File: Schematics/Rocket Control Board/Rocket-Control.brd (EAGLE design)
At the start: 100 x 80 mm, 37 parts

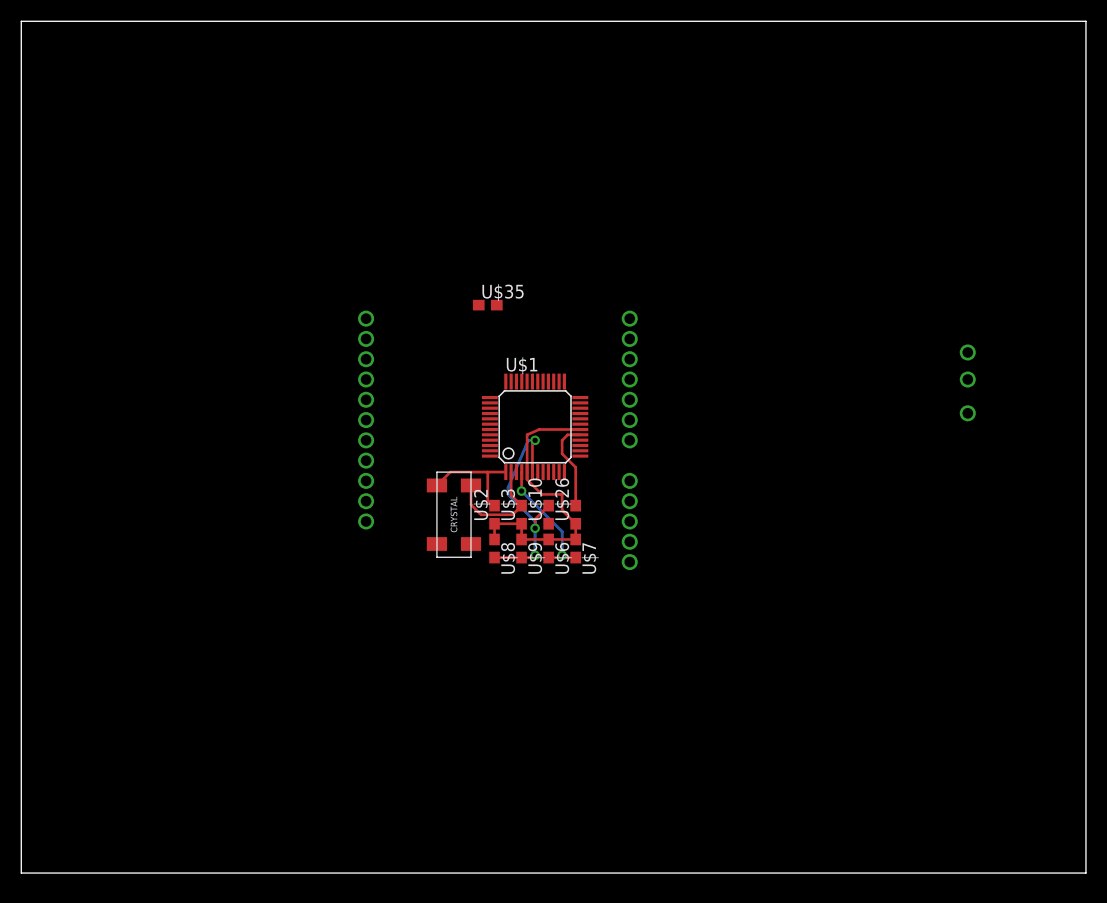
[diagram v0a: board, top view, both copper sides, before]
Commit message: Rocket Control Board Work
Significant changes to rocket control board. Too many to detail.
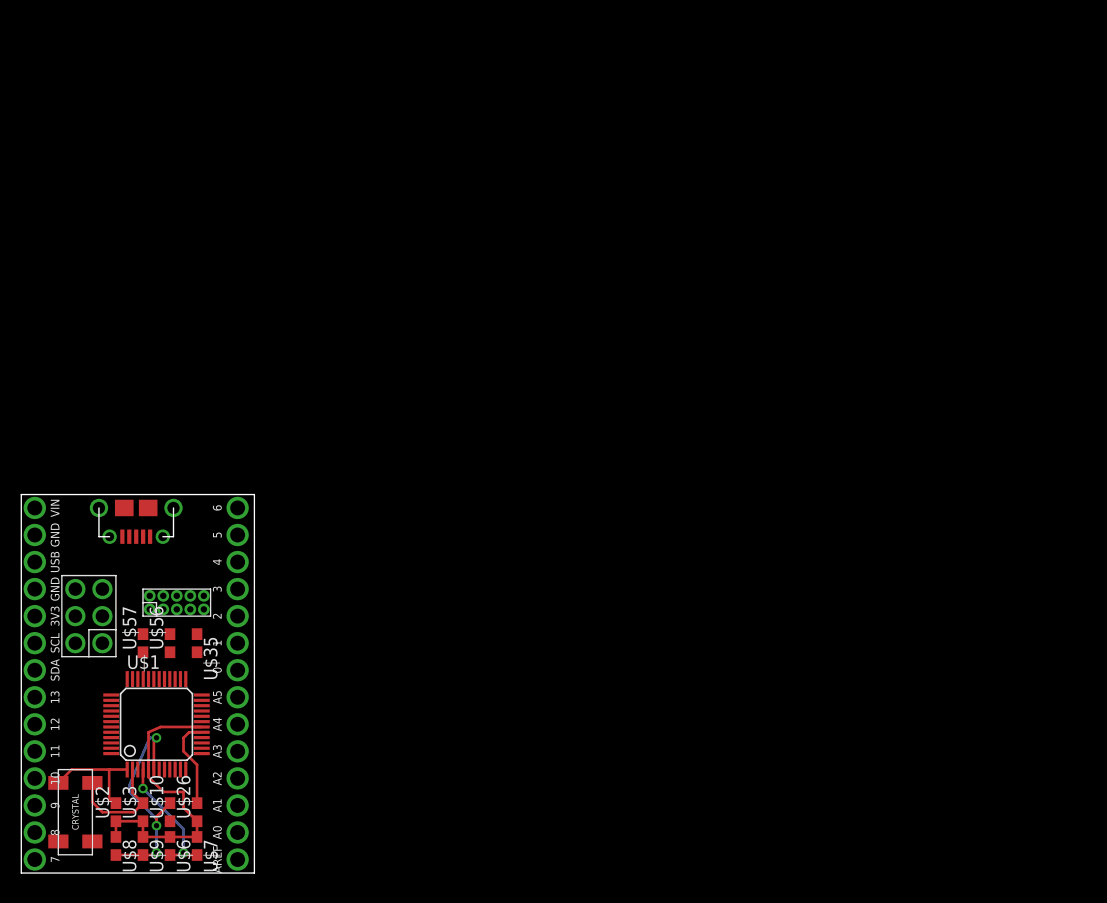
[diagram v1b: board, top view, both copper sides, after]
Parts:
- removed U$11, U$12, U$13, U$14, U$15, U$16, U$17, U$18, U$19, U$20, U$23, U$24, U$25, U$27, U$28, U$29, U$30, U$31, U$32, U$33, U$34, U$36, U$37, U$5: HEADER-HOLE, RocketControlBoard:HEADER-HOLE
- added U$38: 10118194-0001LF:MICRO-USB, RocketControlBoard:10118194-0001LF:MICRO-USB-B
- added U$41: SPI-PORT, RocketControlBoard:SPI-PORT
- added U$56: VDDCORE-CAPACITOR, RocketControlBoard:C0603
- added U$57: VIN-CAPACITOR, RocketControlBoard:C0603
- added U$61: JTAG-MINI, RocketControlBoard:JTAG-MINI
- U$21: value HEADER-HOLE -> HEADER-SIDE-A; device RocketControlBoard:HEADER-HOLE -> RocketControlBoard:HEADER-SIDE-A
- U$22: value HEADER-HOLE -> HEADER-SIDE-B; device RocketControlBoard:HEADER-HOLE -> RocketControlBoard:HEADER-SIDE-B
- moved U$22 88.1 mm to (1.27, 36.8), turned to 90 degrees
- moved U$21 73.6 mm to (20.3, 16.5)
- moved U$1 45.2 mm to (12.7, 14.0)
- moved U$10 45.2 mm to (14.0, 5.71)
- moved U$2 45.2 mm to (8.89, 5.71)
- moved U$26 45.2 mm to (16.5, 5.71)
- moved U$3 45.2 mm to (11.4, 5.71)
- moved U$4 45.2 mm to (5.08, 5.71)
- moved U$6 45.2 mm to (14.0, 2.54)
- moved U$7 45.2 mm to (16.5, 2.54)
- moved U$8 45.2 mm to (8.89, 2.54)
- moved U$9 45.2 mm to (11.4, 2.54)
- moved U$35 41.9 mm to (16.5, 21.6), turned to 270 degrees
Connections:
- new net A5: U$1.47, U$21.A5
- new net RX: U$1.38
- new net SWD-06(RESET): U$1.40, U$61.RESET
- new net SWD-09: U$1.45, U$61.JTAG09
- new net SWD-10: U$1.46, U$61.JTAG10
- new net TX: U$1.37
- new net USB: U$22.USB, U$38.1:VBUS
- new net VDDCORE: U$1.43, U$56.1
- new net VIN: U$1.44, U$22.VIN, U$57.1
- net +3V3: now also U$22.3V3, U$41.VIN, U$61.VIN; no longer U$36.P$1
- net A0: now also U$21.A0; no longer U$5.P$1
- net A1: now also U$21.A1; no longer U$11.P$1
- net A2: now also U$21.A2; no longer U$12.P$1
- net A3: now also U$21.A3; no longer U$13.P$1
- net A4: now also U$21.A4; no longer U$14.P$1
- net AREF: now also U$21.AREF
- net D0-TX: now also U$21.D0; no longer U$18.P$1
- net D1-RX: now also U$21.D1; no longer U$17.P$1
- net D10: now also U$22.D10; no longer U$30.P$1
- net D11: now also U$22.D11; no longer U$32.P$1
- net D12: now also U$22.D12; no longer U$29.P$1
- net D13: now also U$22.D13; no longer U$31.P$1
- net D2: now also U$21.D2; no longer U$20.P$1
- net D3: now also U$21.D3; no longer U$19.P$1
- net D4: now also U$21.D4; no longer U$24.P$1
- net D5: now also U$21.D5; no longer U$25.P$1
- net D6: now also U$21.D6; no longer U$28.P$1
- net D7: now also U$22.D7, U$41.ATN; no longer U$27.P$1
- net D8: now also U$22.D8; no longer U$15.P$1
- net D9: now also U$22.D9; no longer U$16.P$1
- net GND: now also U$1.42, U$22.GND-IN, U$22.GND-OUT, U$38.5:GND, U$41.GND, U$56.2, U$57.2, U$61.GND-1, U$61.GND-2, U$61.GND-3; no longer U$37.P$1
- net MISO: now also U$41.MISO; no longer U$23.P$1
- net MOSI: now also U$41.MOSI; no longer U$21.P$1
- net SCK: now also U$41.SCK; no longer U$22.P$1
- net SCL: now also U$22.SCL; no longer U$34.P$1
- net SDA: now also U$22.SDA; no longer U$33.P$1
- net USB-N: now also U$38.2:D-
- net USB-P: now also U$38.3:D+
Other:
- board size 100 x 80 mm -> 21.9 x 35.5 mm
